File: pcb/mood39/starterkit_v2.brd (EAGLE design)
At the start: 32 x 32 mm, 19 parts, among them IC1 TINY85, IC2 LP2950

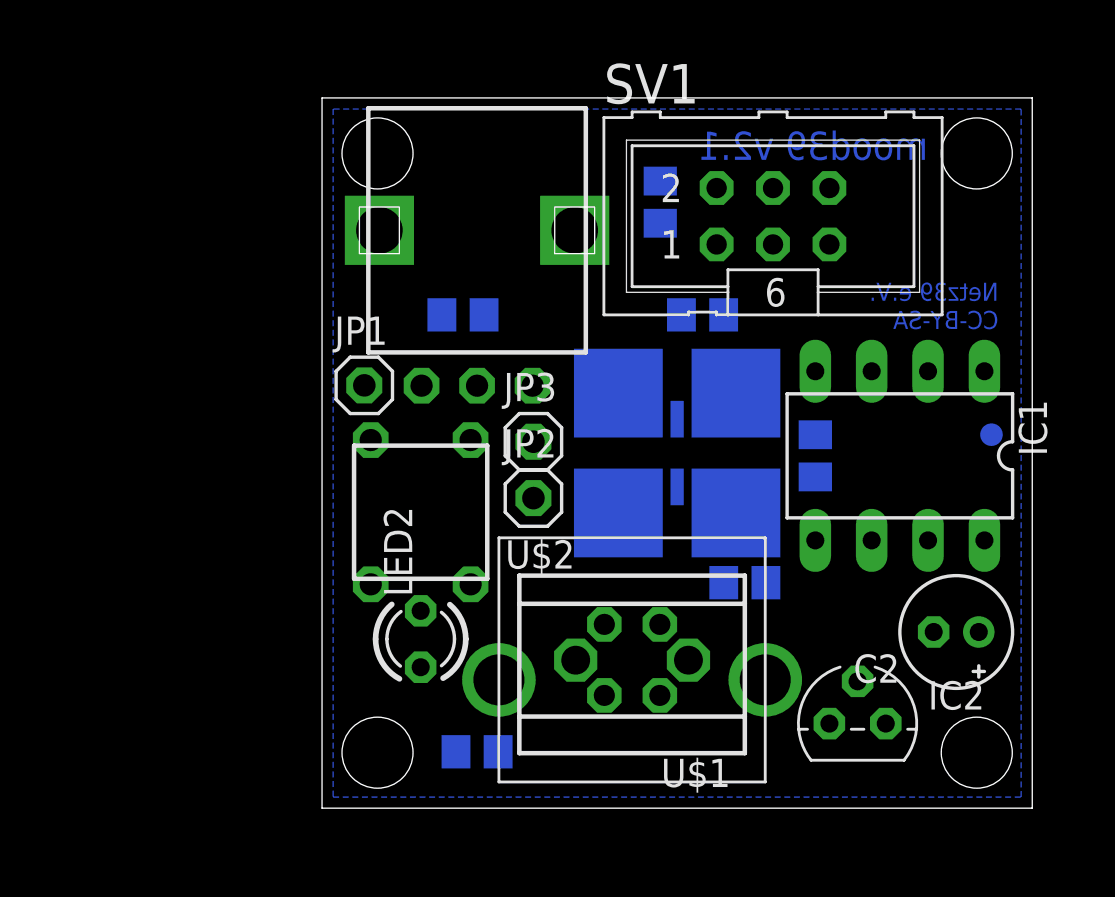
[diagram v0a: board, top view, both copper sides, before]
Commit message: start routing
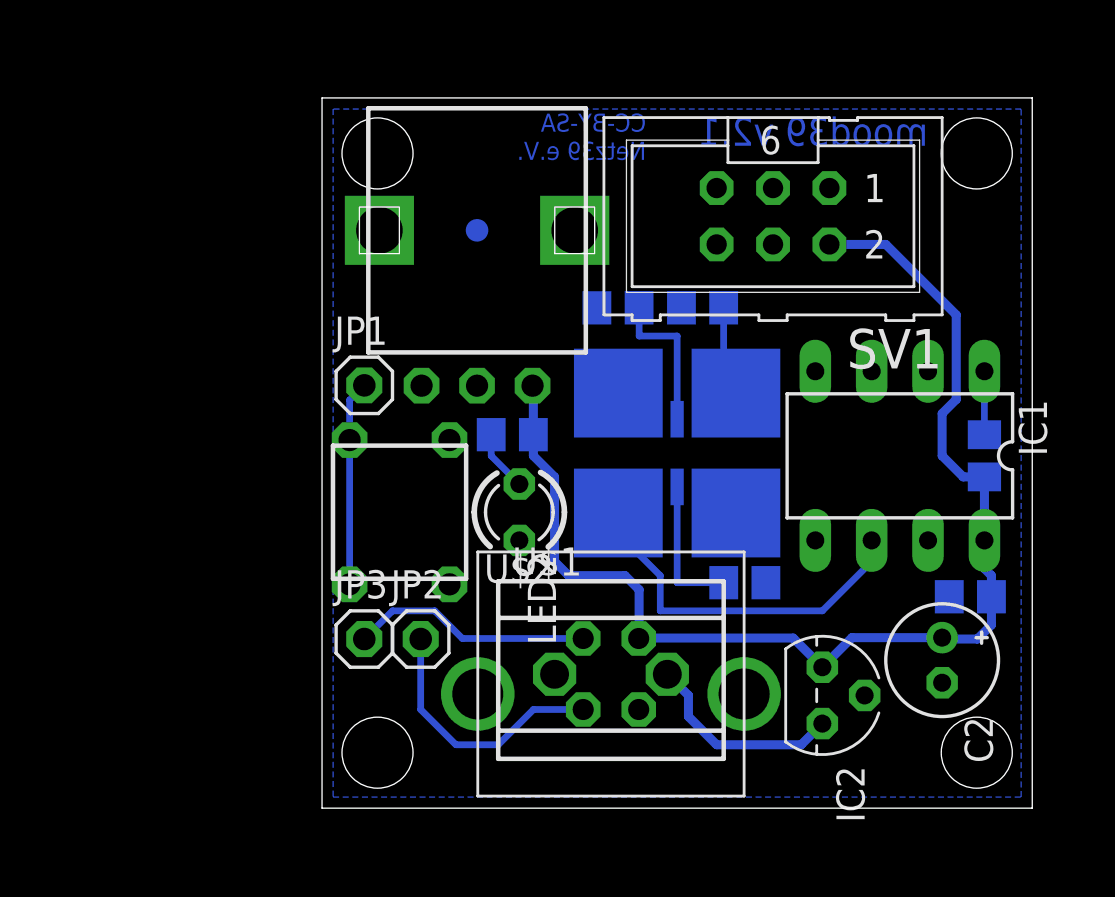
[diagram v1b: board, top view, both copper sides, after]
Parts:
- moved C1 26.2 mm to (29.2, 9.53)
- moved R1 18.5 mm to (29.8, 15.9), turned to 90 degrees
- moved R6 14.4 mm to (8.57, 16.8)
- moved JP3 11.7 mm to (1.91, 7.62)
- moved R4 8.38 mm to (17.1, 22.5), turned to 0 degrees
- moved JP2 8.13 mm to (4.45, 7.62)
- moved LED2 7.24 mm to (8.89, 13.3), turned to 270 degrees
- moved R2 3.82 mm to (13.3, 22.5), turned to 0 degrees
- moved IC2 2.03 mm to (22.5, 5.08), turned to 270 degrees
- moved C2 1.42 mm to (27.9, 6.67), turned to 270 degrees
- moved U$1 1.14 mm to (13.0, 6.03), turned to 0 degrees
- moved U$2 1.14 mm to (13.0, 4.45)
- moved S1 0.95 mm to (3.49, 13.3)
- turned SV1 to 180 degrees
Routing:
- net VCC: track 0.00 -> 54.9 mm
- net MISO: track 0.00 -> 16.6 mm
- net USBD+: track 0.00 -> 11.8 mm
- net USBD-: track 0.00 -> 10.9 mm
- net V+: track 0.00 -> 9.25 mm
- net MOSI: track 0.00 -> 9.24 mm
- net N$5: track 0.00 -> 6.73 mm
- net N$6: track 0.00 -> 6.42 mm
- net N$7: track 0.00 -> 4.40 mm
- net !RESET: track 0.00 -> 2.86 mm
- net N$1: track 0.00 -> 2.75 mm

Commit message: proceed routing, hopefully not a dead end
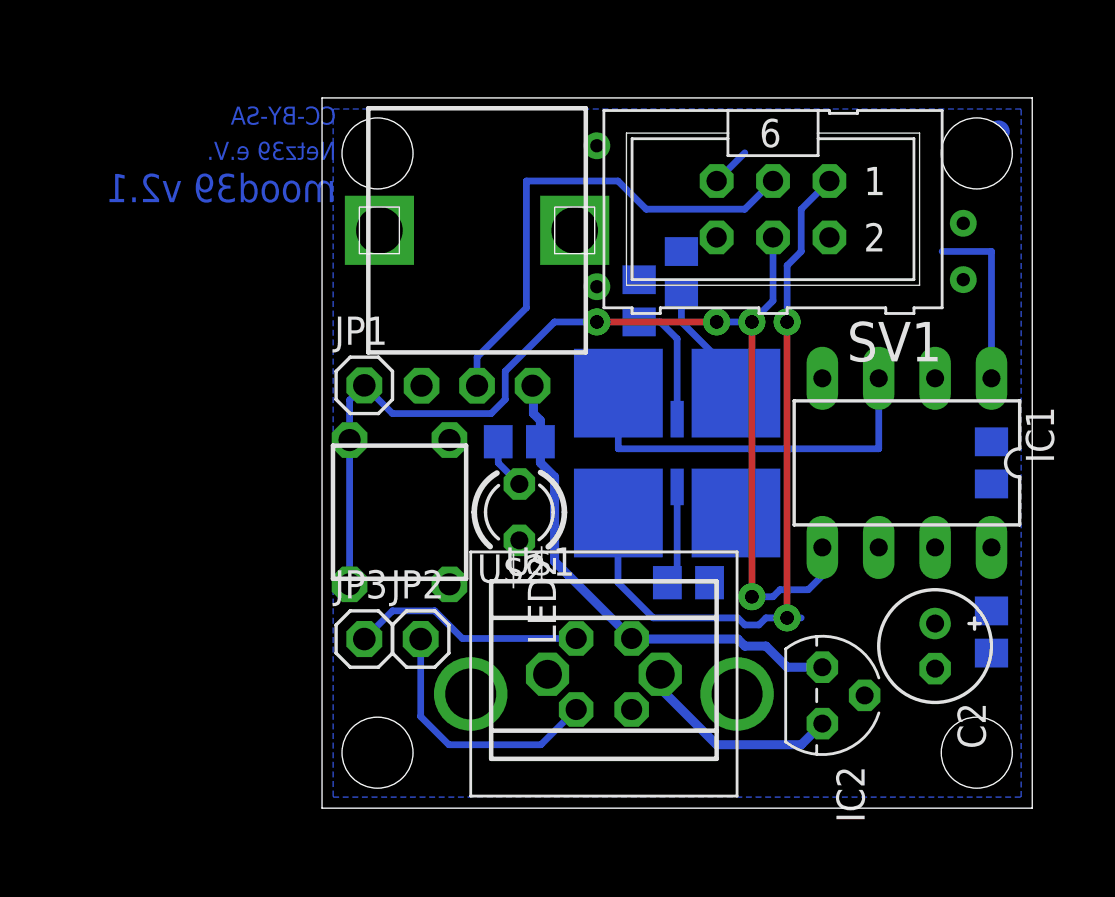
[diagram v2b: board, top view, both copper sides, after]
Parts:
- moved R3 2.54 mm to (16.5, 10.2)
- moved C1 1.85 mm to (30.2, 7.94), turned to 270 degrees
- moved R4 1.85 mm to (16.2, 24.1), turned to 90 degrees
- moved R2 1.00 mm to (14.3, 22.9), turned to 90 degrees
- moved C2 0.71 mm to (27.6, 7.30)
- moved R1 0.45 mm to (30.2, 15.6)
- moved IC1 0.45 mm to (26.4, 15.6)
- moved R6 0.45 mm to (8.89, 16.5)
- moved U$1 0.32 mm to (12.7, 6.03)
- moved U$2 0.32 mm to (12.7, 4.45)
- moved SV1 0.32 mm to (20.3, 27.0)
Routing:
- net MOSI: track 9.24 -> 51.1 mm, vias 0 -> 4
- net VCC: track 54.9 -> 22.4 mm
- net SCK: track 0.00 -> 22.3 mm
- net PB4: track 0.00 -> 17.4 mm
- net MISO: track 16.6 -> 32.8 mm, vias 0 -> 2
- net !RESET: track 2.86 -> 9.73 mm
- net N$6: track 6.42 -> 4.50 mm
- net N$7: track 4.40 -> 5.50 mm
- net N$5: track 6.73 -> 5.65 mm
